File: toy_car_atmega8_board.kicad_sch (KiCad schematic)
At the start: 15 parts, among them J1 Conn_01x06_Pin, J2 Conn_01x08_Pin, J3 Conn_01x06_Pin, J4 Conn_01x06_Pin, J5 Conn_01x02_Pin, SW1 SW_Push, U1 ATmega8A-P, Y1 Crystal

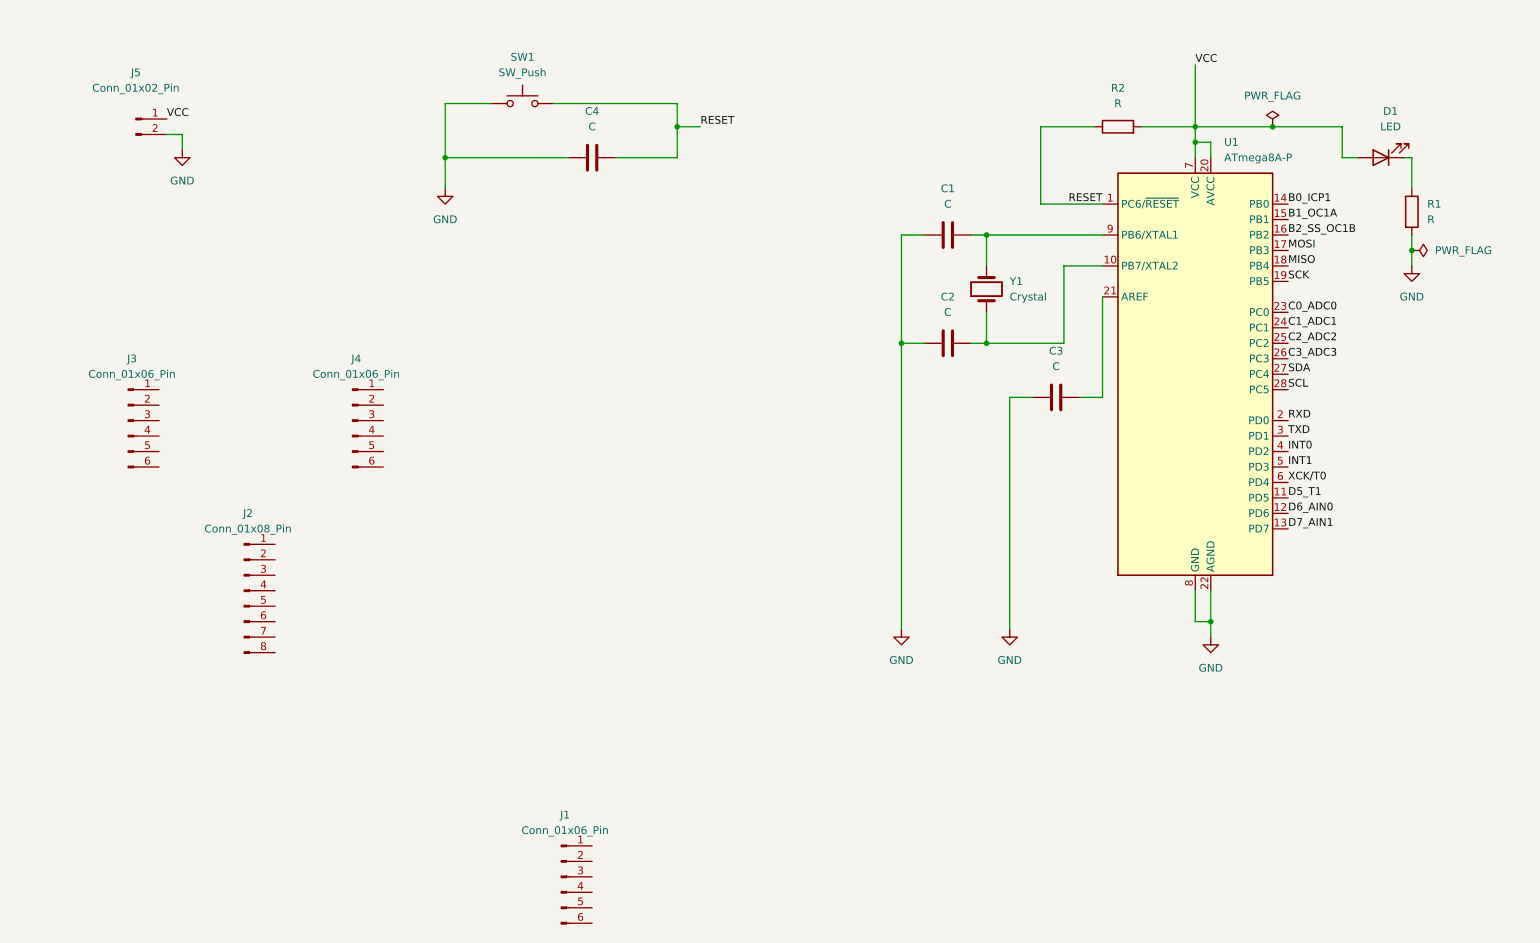
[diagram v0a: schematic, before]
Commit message: Added footprints and value, checked electrical connections. All good
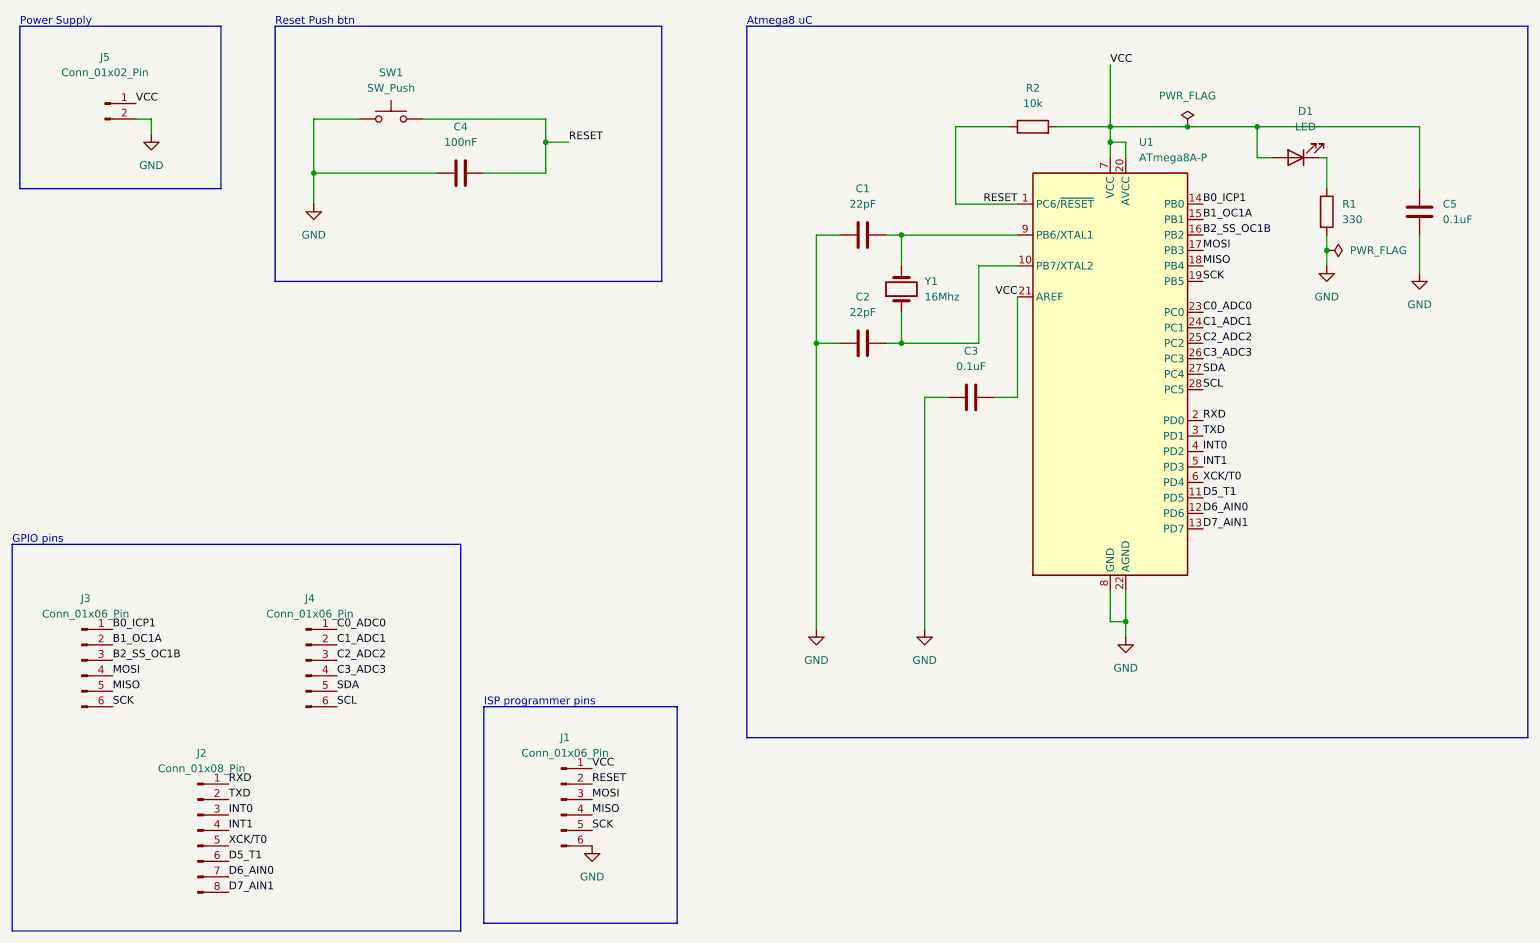
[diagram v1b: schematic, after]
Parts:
- added C5: 0.1uF, Capacitor_THT:C_Disc_D3.8mm_W2.6mm_P2.50mm, symbol Device:C
- C1, C2: value C -> 22pF; footprint (none) -> Capacitor_THT:C_Disc_D3.8mm_W2.6mm_P2.50mm
- C3: value C -> 0.1uF; footprint (none) -> Capacitor_THT:C_Disc_D3.8mm_W2.6mm_P2.50mm
- C4: value C -> 100nF; footprint (none) -> Capacitor_THT:C_Disc_D3.8mm_W2.6mm_P2.50mm
- D1: footprint (none) -> LED_THT:LED_D3.0mm
- J1, J3, J4: footprint (none) -> Connector_PinHeader_2.54mm:PinHeader_1x06_P2.54mm_Vertical
- J2: footprint (none) -> Connector_PinHeader_2.54mm:PinHeader_1x08_P2.54mm_Vertical
- J5: footprint (none) -> Connector_PinHeader_2.54mm:PinHeader_1x02_P2.54mm_Vertical
- R1: value R -> 330; footprint (none) -> Resistor_THT:R_Axial_DIN0207_L6.3mm_D2.5mm_P7.62mm_Horizontal
- R2: value R -> 10k; footprint (none) -> Resistor_THT:R_Axial_DIN0207_L6.3mm_D2.5mm_P7.62mm_Horizontal
- SW1: footprint (none) -> Button_Switch_THT:SW_PUSH_6mm
- Y1: value Crystal -> 16Mhz; footprint (none) -> Crystal:Crystal_HC18-U_Vertical
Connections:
- net B0_ICP1: now also J3.1 (Pin_1)
- net B1_OC1A: now also J3.2 (Pin_2)
- net B2_SS_OC1B: now also J3.3 (Pin_3)
- net C0_ADC0: now also J4.1 (Pin_1)
- net C1_ADC1: now also J4.2 (Pin_2)
- net C2_ADC2: now also J4.3 (Pin_3)
- net C3_ADC3: now also J4.4 (Pin_4)
- net D5_T1: now also J2.6 (Pin_6)
- net D6_AIN0: now also J2.7 (Pin_7)
- net D7_AIN1: now also J2.8 (Pin_8)
- net GND: now also J1.6 (Pin_6), C5.1
- net INT0: now also J2.3 (Pin_3)
- net INT1: now also J2.4 (Pin_4)
- net MISO: now also J1.4 (Pin_4), J3.5 (Pin_5)
- net MOSI: now also J1.3 (Pin_3), J3.4 (Pin_4)
- net RESET: now also J1.2 (Pin_2)
- net RXD: now also J2.1 (Pin_1)
- net SCK: now also J1.5 (Pin_5), J3.6 (Pin_6)
- net SCL: now also J4.6 (Pin_6)
- net SDA: now also J4.5 (Pin_5)
- net TXD: now also J2.2 (Pin_2)
- net VCC: now also C3.2, J1.1 (Pin_1), U1.21 (AREF), C5.2
- net XCK/T0: now also J2.5 (Pin_5)
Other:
- note added: "Atmega8 uC"
- note added: "GPIO pins"
- note added: "ISP programmer pins"
- note added: "Power Supply"
- note added: "Reset Push btn"
- company: (none) -> R.K hobbyst
- title: (none) -> Toy car microcontroller
- moved on the sheet: C1, C2, C3, C4, D1, J1, J2, J3, J4, J5, R1, R2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
